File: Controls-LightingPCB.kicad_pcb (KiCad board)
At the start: 2 copper layers, 63.5 x 114.3 mm, 65 parts, among them J1 MinionConn, J2 Backup, SW1 HAZARD, SW2 CRUISE_SET, SW3 CRUISE, SW4 F/R_SW, SW5 HEADLIGHT_SW, SW6 BACKUP_SW, SW7 TURN_SIGNAL_SW, SW8 REGEN_SW, U1 LTC6820, U2 HX1188FNL, U3 MCP23S17_SO, U4 RI3-1205S, U5 NCP1117-3.3_SOT223

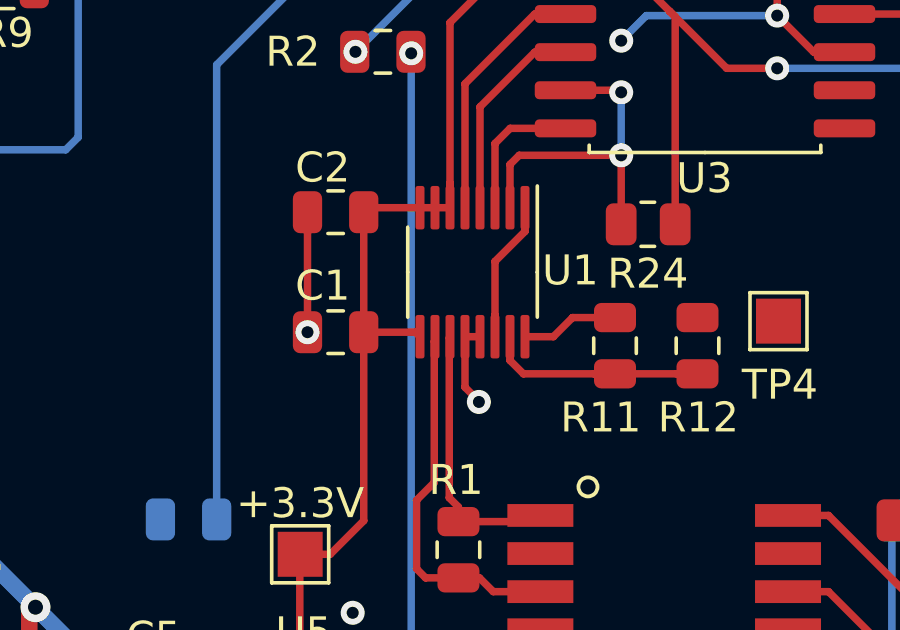
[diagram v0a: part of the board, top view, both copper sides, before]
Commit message: Adds the gerbers
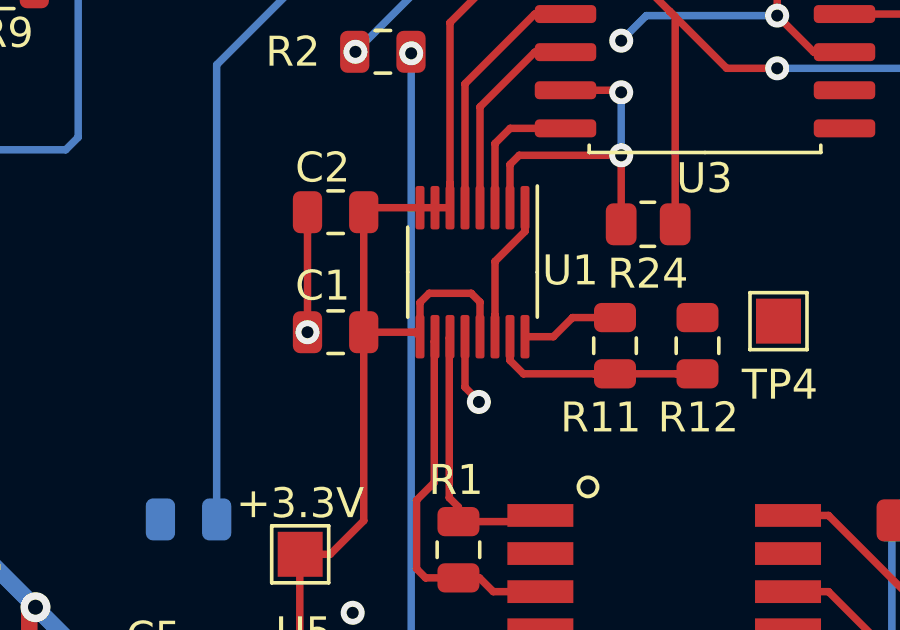
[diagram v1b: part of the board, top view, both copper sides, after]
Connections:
- U1 pad 13: GND -> +3V3
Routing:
- net +3V3: track 273.4 -> 277.9 mm
- net GND: track 48.0 -> 47.5 mm
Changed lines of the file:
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@@
     (thickness 1.6)
     (drawings 40)
-    (tracks 437)
+    (tracks 441)
     (zones 0)
     (modules 65)
@@
       (net 11 GND))
     (pad 13 smd roundrect (at 2.15 -0.25 270) (size 1.45 0.3) (layers F.Cu F.Paste F.Mask) (roundrect_rratio 0.25)
-      (net 11 GND))
+      (net 10 +3V3))
     (pad 14 smd roundrect (at 2.15 -0.75 270) (size 1.45 0.3) (layers F.Cu F.Paste F.Mask) (roundrect_rratio 0.25)
       (net 11 GND))
@@
   (segment (start 159.61338 118.19662) (end 161.51676 120.1) (width 0.25) (layer F.Cu) (net 10))
   (segment (start 157.16846 115.7517) (end 159.61338 118.19662) (width 0.25) (layer F.Cu) (net 10))
+  (segment (start 153.29346 129.0467) (end 153.29346 127.89346) (width 0.25) (layer F.Cu) (net 10))
+  (segment (start 153.29346 127.89346) (end 153 127.6) (width 0.25) (layer F.Cu) (net 10))
+  (segment (start 153 127.6) (end 151.6 127.6) (width 0.25) (layer F.Cu) (net 10))
+  (segment (start 151.29346 127.90654) (end 151.29346 129.0467) (width 0.25) (layer F.Cu) (net 10))
+  (segment (start 151.6 127.6) (end 151.29346 127.90654) (width 0.25) (layer F.Cu) (net 10))
   (segment (start 153.79346 128.3217) (end 153.79346 129.0467) (width 0.25) (layer F.Cu) (net 11))
   (segment (start 153.79346 126.537402) (end 153.79346 128.3217) (width 0.25) (layer F.Cu) (net 11))
   (segment (start 154.79346 125.537402) (end 153.79346 126.537402) (width 0.25) (layer F.Cu) (net 11))
   (segment (start 154.79346 124.7467) (end 154.79346 125.537402) (width 0.25) (layer F.Cu) (net 11))
-  (segment (start 153.29346 129.0467) (end 152.79346 129.0467) (width 0.25) (layer F.Cu) (net 11))
   (segment (start 152.79346 130.73154) (end 153.256 131.19408) (width 0.25) (layer F.Cu) (net 11))
   (segment (start 147.54346 124.8967) (end 147.54346 125.5967) (width 0.25) (layer F.Cu) (net 11))
